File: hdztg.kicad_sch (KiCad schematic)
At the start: 8 parts, among them J1 20374-R20E-31, Q1 2N7002KDW 72K

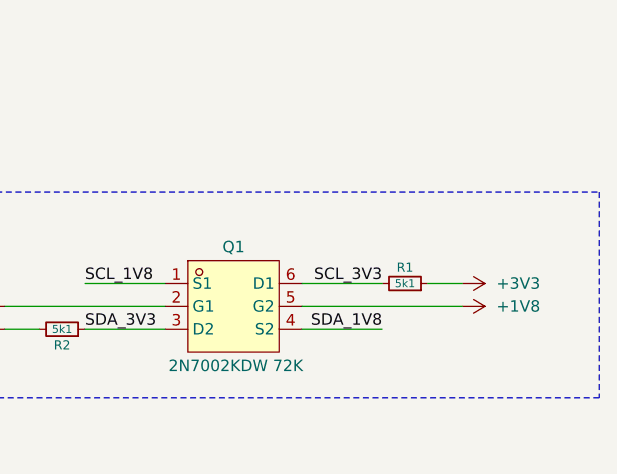
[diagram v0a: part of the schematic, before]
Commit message: update pcb
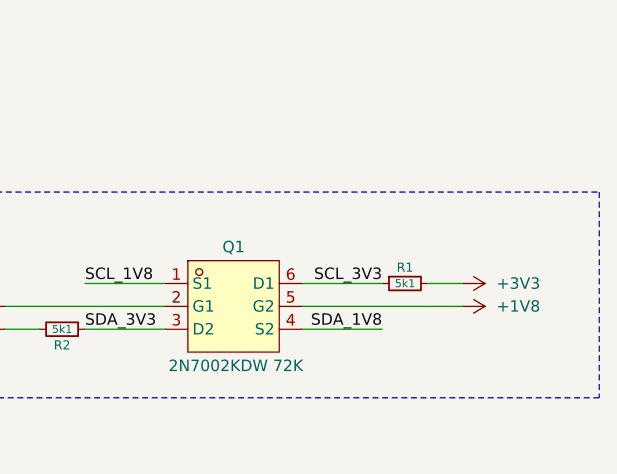
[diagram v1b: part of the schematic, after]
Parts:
- FPC1: Manufacturer Part (none) -> FPC-05FB-24PH20; Supplier Link (none) -> https://lcsc.com/product-detail/FFC-FPC-Flat-Flexible-Conne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
- J1: Availability In Stock -> (none); Check_prices https://www.snapeda.com/parts/20374-R20E-31/I-PEX/view-part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 -> (none); Description_1 20 POS Right Angle SMD 0.4 mm pitch vertical mating type mi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 -> (none); DigiKey Part (none) -> 5378-20374-R20E-31TR-ND; MANUFACTURER I-PEX -> (none); MF I-PEX -> (none); MP 20374-R20E-31 -> (none); Manufacturer (none) -> I-PEX; Manufacturer Product Number (none) -> 20374-R20E-31; PARTREV 24 -> (none); Package None -> (none); Price None -> (none); STANDARD Manufacturer Recommendation -> (none); SnapEDA_Link https://www.snapeda.com/parts/20374-R20E-31/I-PEX/view-part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 -> (none); Supplier Link (none) -> https://www.digikey.com/en/products/detail/i-pex/20374-R20E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
- Q1: Manufacturer Part (none) -> 2N7002KDW; Supplier Link (none) -> https://lcsc.com/product-detail/MOSFETs_CBI-2N7002KDW_C2919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
- R1, R2: LCSC Part (none) -> C274341; Manufacturer Part (none) -> RC0201FR-075K1L; Supplier Link (none) -> https://lcsc.com/product-detail/Chip-Resistor-Surface-Mount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
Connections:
- net +3V3: now also R1.2; no longer R1.1
- net SCL_3V3: now also R1.1; no longer R1.2
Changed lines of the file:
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@@
 			)
 		)
-		(property "Datasheet" ""
+		(property "Datasheet" "https://www.i-pex.com/sites/default/files/downloads/pdf/CATALOG_CABLINE-SS_E.pdf"
 			(at 35.56 62.23 0)
 			(effects
@@
 			)
 		)
-		(property "Description" ""
+		(property "Description" "20 POS Right Angle SMD 0.4 mm pitch vertical mating type micro-coaxial connector with friction lock CABLINE SS Receptacle"
 			(at 35.56 62.23 0)
 			(effects
@@
 			)
 		)
-		(property "MF" "I-PEX"
+		(property "Manufacturer Product Number" "20374-R20E-31"
 			(at 35.56 62.23 0)
 			(effects
@@
 			)
 		)
-		(property "Description_1" "20 POS Right Angle SMD 0.4 mm pitch vertical mating type micro-coaxial connector with friction lock CABLINE SS Receptacle"
+		(property "Manufacturer" "I-PEX"
 			(at 35.56 62.23 0)
 			(effects
@@
 			)
 		)
-		(property "Package" "None"
+		(property "DigiKey Part" "5378-20374-R20E-31TR-ND"
 			(at 35.56 62.23 0)
 			(effects
@@
 					(size 1.27 1.27)
 				)
-				(justify bottom)
-				(hide yes)
-			)
-		)
-		(property "Price" "None"
+				(hide yes)
+			)
+		)
+		(property "Supplier Link" "https://www.digikey.com/en/products/detail/i-pex/20374-R20E-31/24394701"
 			(at 35.56 62.23 0)
 			(effects
@@
 					(size 1.27 1.27)
 				)
-				(justify bottom)
-				(hide yes)
-			)
-		)
-		(property "Check_prices" "https://www.snapeda.com/parts/20374-R20E-31/I-PEX/view-part/?ref=eda"
-			(at 35.56 62.23 0)
-			(effects
-				(font
-					(size 1.27 1.27)
-				)
-				(justify bottom)
-				(hide yes)
-			)
-		)
-		(property "STANDARD" "Manufacturer Recommendation"
-			(at 35.56 62.23 0)
-			(effects
-				(font
-					(size 1.27 1.27)
-				)
-				(justify bottom)
-				(hide yes)
-			)
-		)
-		(property "PARTREV" "24"
-			(at 35.56 62.23 0)
-			(effects
-				(font
-					(size 1.27 1.27)
-				)
-				(justify bottom)
-				(hide yes)
-			)
-		)
-		(property "SnapEDA_Link" "https://www.snapeda.com/parts/20374-R20E-31/I-PEX/view-part/?ref=snap"
-			(at 35.56 62.23 0)
-			(effects
-				(font
-					(size 1.27 1.27)
-				)
-				(justify bottom)
-				(hide yes)
-			)
-		)
-		(property "MP" "20374-R20E-31"
-			(at 35.56 62.23 0)
-			(effects
-				(font
-					(size 1.27 1.27)
-				)
-				(justify bottom)
-				(hide yes)
-			)
-		)
-		(property "Availability" "In Stock"
-			(at 35.56 62.23 0)
-			(effects
-				(font
-					(size 1.27 1.27)
-				)
-				(justify bottom)
-				(hide yes)
-			)
-		)
-		(property "MANUFACTURER" "I-PEX"
-			(at 35.56 62.23 0)
-			(effects
-				(font
-					(size 1.27 1.27)
-				)
-				(justify bottom)
 				(hide yes)
 			)
@@
 			)
 		)
+		(property "Manufacturer Part" "2N7002KDW"
+			(at 151.13 88.9 0)
+			(effects
+				(font
+					(size 1.27 1.27)
+				)
+				(hide yes)
+			)
+		)
 		(property "LCSC Part" "C2919800"
 			(at 151.13 101.6 0)
+			(effects
+				(font
+					(size 1.27 1.27)
+				)
+				(hide yes)
+			)
+		)
+		(property "Supplier Link" "https://lcsc.com/product-detail/MOSFETs_CBI-2N7002KDW_C2919800.html?s_z=n_2N7002KDW"
+			(at 151.13 88.9 0)
 			(effects
 				(font
@@
 	)
 	(symbol
+		(lib_id "Device:R_Small")
+		(at 170.18 86.36 90)
+		(mirror x)
+		(unit 1)
+		(exclude_from_sim no)
+		(in_bom yes)
+		(on_board yes)
+		(dnp no)
+		(property "Reference" "R1"
+			(at 170.18 84.582 90)
+			(effects
+				(font
+					(size 1.016 1.016)
+				)
+			)
+		)
+		(property "Value" "5k1"
+			(at 170.18 86.36 90)
+			(effects
+				(font
+					(size 0.889 0.889)
+				)
+			)
+		)
+		(property "Footprint" "Resistor_SMD:R_0201_0603Metric"
+			(at 170.18 86.36 0)
+			(effects
+				(font
+					(size 1.27 1.27)
+				)
+				(hide yes)
+			)
+		)
+		(property "Datasheet" "https://lcsc.com/datasheet/lcsc_datasheet_2506161045_YAGEO-RC0201FR-075K1L_C274341.pdf"
+			(at 170.18 86.36 0)
+			(effects
+				(font
+					(size 1.27 1.27)
+				)
+				(hide yes)
+			)
+		)
+		(property "Description" "Resistor, small symbol"
+			(at 170.18 86.36 0)
+			(effects
+				(font
+					(size 1.27 1.27)
+				)
+				(hide yes)
+			)
+		)
+		(property "Manufacturer Part" "RC0201FR-075K1L"
+			(at 170.18 86.36 90)
+			(effects
+				(font
+					(size 1.27 1.27)
+				)
+				(hide yes)
+			)
+		)
+		(property "LCSC Part" "C274341"
+			(at 170.18 86.36 90)
+			(effects
+				(font
+					(size 1.27 1.27)
+				)
+				(hide yes)
+			)
+		)
+		(property "Supplier Link" "https://lcsc.com/product-detail/Chip-Resistor-Surface-Mount_YAGEO-RC0201FR-075K1L_C274341.html"
+			(at 170.18 86.36 90)
+			(effects
+				(font
+					(size 1.27 1.27)
+				)
+				(hide yes)
+			)
+		)
+		(pin "1"
+		)
+		(pin "2"
+		)
+		(instances
+			(project "hdztg"
+				(path "/5fa3be86-0836-40c5-8497-58cbc35ea59a"
+					(reference "R1")
+					(unit 1)
+				)
+			)
+		)
+	)
+	(symbol
 		(lib_id "power:GND")
 		(at 58.42 41.91 90)
@@
 				(path "/5fa3be86-0836-40c5-8497-58cbc35ea59a"
 					(reference "#PWR015")
-					(unit 1)
-				)
-			)
-		)
-	)
-	(symbol
-		(lib_id "Device:R_Small")
-		(at 170.18 86.36 270)
-		(mirror x)
-		(unit 1)
-		(exclude_from_sim no)
-		(in_bom yes)
-		(on_board yes)
-		(dnp no)
-		(property "Reference" "R1"
-			(at 170.18 84.582 90)
-			(effects
-				(font
-					(size 1.016 1.016)
-				)
-			)
-		)
-		(property "Value" "5k1"
-			(at 170.18 86.36 90)
-			(effects
-				(font
-					(size 0.889 0.889)
-				)
-			)
-		)
-		(property "Footprint" "Resistor_SMD:R_0201_0603Metric"
-			(at 170.18 86.36 0)
-			(effects
-				(font
-					(size 1.27 1.27)
-				)
-				(hide yes)
-			)
-		)
-		(property "Datasheet" "~"
-			(at 170.18 86.36 0)
-			(effects
-				(font
-					(size 1.27 1.27)
-				)
-				(hide yes)
-			)
-		)
-		(property "Description" "Resistor, small symbol"
-			(at 170.18 86.36 0)
-			(effects
-				(font
-					(size 1.27 1.27)
-				)
-				(hide yes)
-			)
-		)
-		(pin "1"
-		)
-		(pin "2"
-		)
-		(instances
-			(project "hdztg"
-				(path "/5fa3be86-0836-40c5-8497-58cbc35ea59a"
-					(reference "R1")
 					(unit 1)
 				)
@@
 			)
 		)
-		(property "Datasheet" "~"
+		(property "Datasheet" "https://lcsc.com/datasheet/lcsc_datasheet_2506161045_YAGEO-RC0201FR-075K1L_C274341.pdf"
 			(at 132.08 91.44 0)
 			(effects
@@
 			)
 		)
+		(property "Manufacturer Part" "RC0201FR-075K1L"
+			(at 132.08 91.44 90)
+			(effects
+				(font
+					(size 1.27 1.27)
+				)
+				(hide yes)
+			)
+		)
+		(property "LCSC Part" "C274341"
+			(at 132.08 91.44 90)
+			(effects
+				(font
+					(size 1.27 1.27)
+				)
+				(hide yes)
+			)
+		)
+		(property "Supplier Link" "https://lcsc.com/product-detail/Chip-Resistor-Surface-Mount_YAGEO-RC0201FR-075K1L_C274341.html"
+			(at 132.08 91.44 90)
+			(effects
+				(font
+					(size 1.27 1.27)
+				)
+				(hide yes)
+			)
+		)
 		(pin "1"
 		)
@@
 			)
 		)
-		(property "Datasheet" ""
+		(property "Datasheet" "https://lcsc.com/datasheet/lcsc_datasheet_2411121000_XUNPU-FPC-05FB-24PH20_C2856831.pdf"
 			(at 88.9 63.5 0)
 			(effects
@@
 			)
 		)
-		(property "Description" ""
+		(property "Description" "Hinged Lid -25℃~+85℃ 24P Double-Sided Contacts, Top and Bottom Entry Surface Mount, Right Angle 0.5mm SMD,P=0.5mm,Surface Mount,Right Angle FFC, FPC (Flat Flexible) Connector Assemblies ROHS"
+			(at 88.9 63.5 0)
+			(effects
+				(font
+					(size 1.27 1.27)
+				)
+				(hide yes)
+			)
+		)
+		(property "Manufacturer Part" "FPC-05FB-24PH20"
 			(at 88.9 63.5 0)
 			(effects
@@
 			(effects
 				(font
+					(size 1.27 1.27)
+				)
+				(hide yes)
+			)
+		)
+		(property "Supplier Link" "https://lcsc.com/product-detail/FFC-FPC-Flat-Flexible-Connector-Assemblies_XUNPU-FPC-05FB-24PH20_C2856831.html?s_z=n_FPC-05FB-24PH20"
+			(at 88.9 63.5 0)
+			(effects
+				(font
